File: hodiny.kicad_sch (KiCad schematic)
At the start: 58 parts, among them U1 DS1302+, U10 4511, U11 4511, U12 4511, U2 4511, U8 4511, U9 4511, Y1 32.768kHz

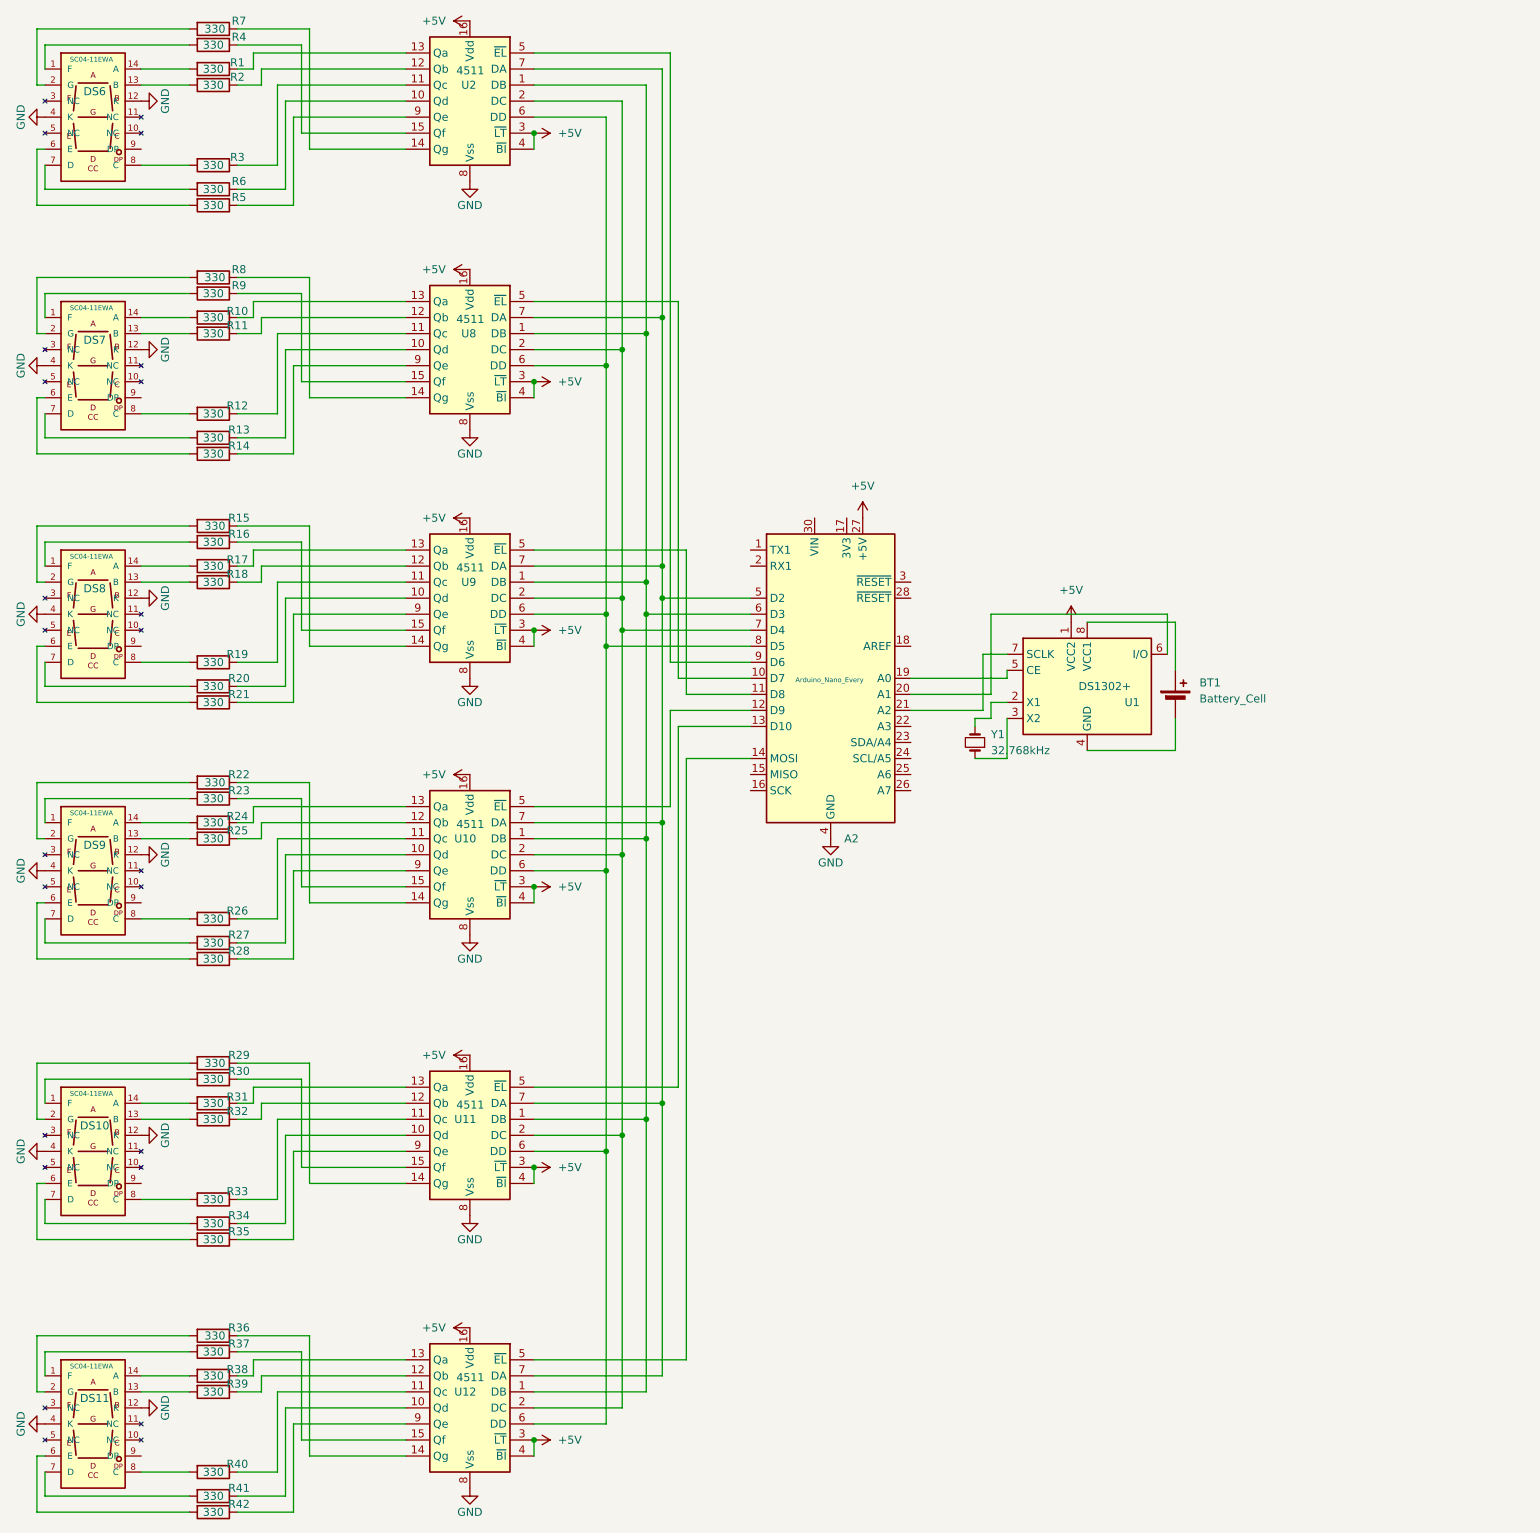
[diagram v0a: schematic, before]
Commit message: Add files via upload
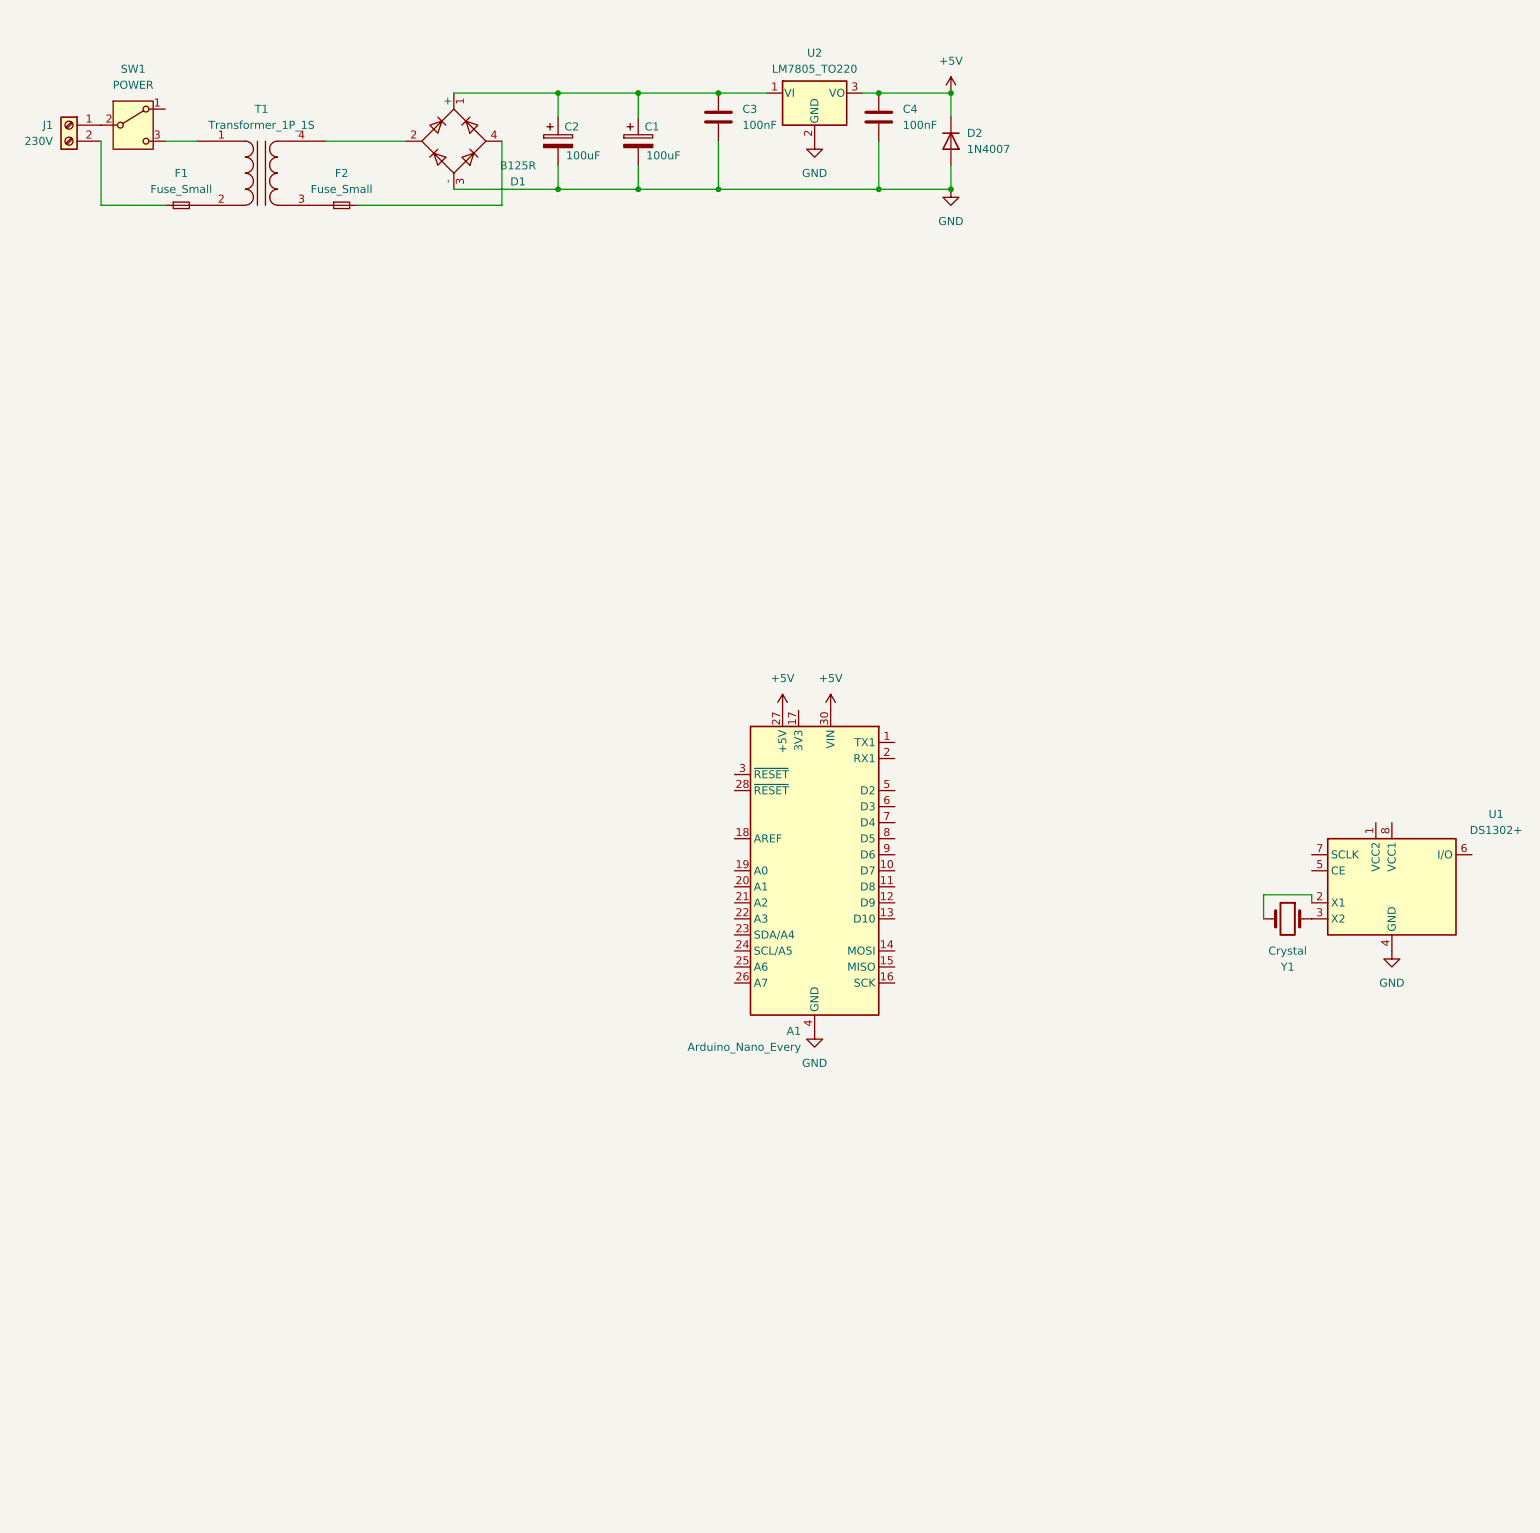
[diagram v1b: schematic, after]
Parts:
- removed A2: Arduino_Nano_Every, Module:Arduino_Nano, symbol MCU_Module:Arduino_Nano_Every
- removed BT1: Battery_Cell, Battery:BatteryHolder_ComfortableElectronic_CH273-2450_1x2450, symbol Device:Battery_Cell
- removed DS10, DS11, DS6, DS7, DS8, DS9: SC04-11EWA, SC04-11EWA:SC04-11EWA_THT, symbol SC04-11EWA:SC04-11EWA
- removed R1, R10, R11, R12, R13, R14, R15, R16, R17, R18, R19, R2, R20, R21, R22, R23, R24, R25, R26, R27, R28, R29, R3, R30, R31, R32, R33, R34, R35, R36, R37, R38, R39, R4, R40, R41, R42, R5, R6, R7, R8, R9: 330, Resistor_THT:R_Axial_DIN0411_L9.9mm_D3.6mm_P15.24mm_Horizontal, symbol Device:R
- removed U10, U11, U12, U2, U8, U9: 4511, Package_DIP:DIP-16_W7.62mm_Socket_LongPads, symbol 4xxx_IEEE:4511
- removed Y1: 32.768kHz, Crystal:Crystal_C26-LF_D2.1mm_L6.5mm_Horizontal, symbol PCM_SparkFun-Clock:Crystal_32.768kHz_3.2x1.5mm
- added A1: Arduino_Nano_Every, Module:Arduino_Nano, symbol MCU_Module:Arduino_Nano_Every
- added C1, C2: 100uF, Package_DFN_QFN:WDFN-10-1EP_3x3mm_P0.5mm_EP1.8x2.5mm, symbol Device:C_Polarized
- added C3, C4: 100nF, Diode_THT:Diode_Bridge_Round_D9.0mm, symbol Device:C
- added D1: B125R, Diode_THT:Diode_Bridge_Round_D9.0mm, symbol Diode_Bridge:B125R
- added D2: 1N4007, Diode_THT:D_DO-41_SOD81_P12.70mm_Horizontal, symbol Diode:1N4007
- added F1, F2: Fuse_Small, Package_QFP:LQFP-100_14x14mm_P0.5mm, symbol Device:Fuse_Small
- added J1: 230V, Package_DFN_QFN:QFN-20-1EP_5x5mm_P0.65mm_EP3.35x3.35mm, symbol Connector:Screw_Terminal_01x02
- added SW1: POWER, Button_Switch_THT:SW_NKK_GW12LJP, symbol Switch:SW_SPDT
- added T1: Transformer_1P_1S, symbol Device:Transformer_1P_1S
- added U2: LM7805_TO220, Package_TO_SOT_THT:TO-220-3_Vertical, symbol Regulator_Linear:LM7805_TO220
- added Y1: Crystal, Crystal:Crystal_AT310_D3.0mm_L10.0mm_Vertical, symbol Device:Crystal
- U1: footprint Package_DIP:DIP-8_W7.62mm_Socket_LongPads -> Package_DIP:DIP-8_W7.62mm_LongPads
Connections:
- net +5V: now also A1.27 (+5V), A1.30 (VIN), C4.1, D2.1 (K), U2.3 (VO); no longer U1.1 (VCC2)
- net GND: now also U1.4 (GND), A1.29 (GND), A1.4 (GND), C1.2, C2.2, C3.2, C4.2, D1.3 (-), D2.2 (A), U2.2 (GND)
- net at U1.2 (X1): now also Y1.2
- net at U1.3 (X2): now also Y1.1
- new net: C1.1, C2.1, C3.1, D1.1 (+), U2.1 (VI)
- new net: F1.1, J1.2 (Pin_2)
- new net: F1.2, T1.2 (AB)
- new net: J1.1 (Pin_1), SW1.2 (B)
- new net: SW1.3 (C), T1.1 (AA)
- new net: F2.1, T1.3 (SA)
- new net: D1.4, F2.2
- new net: D1.2, T1.4 (SB)

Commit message: Add files via upload
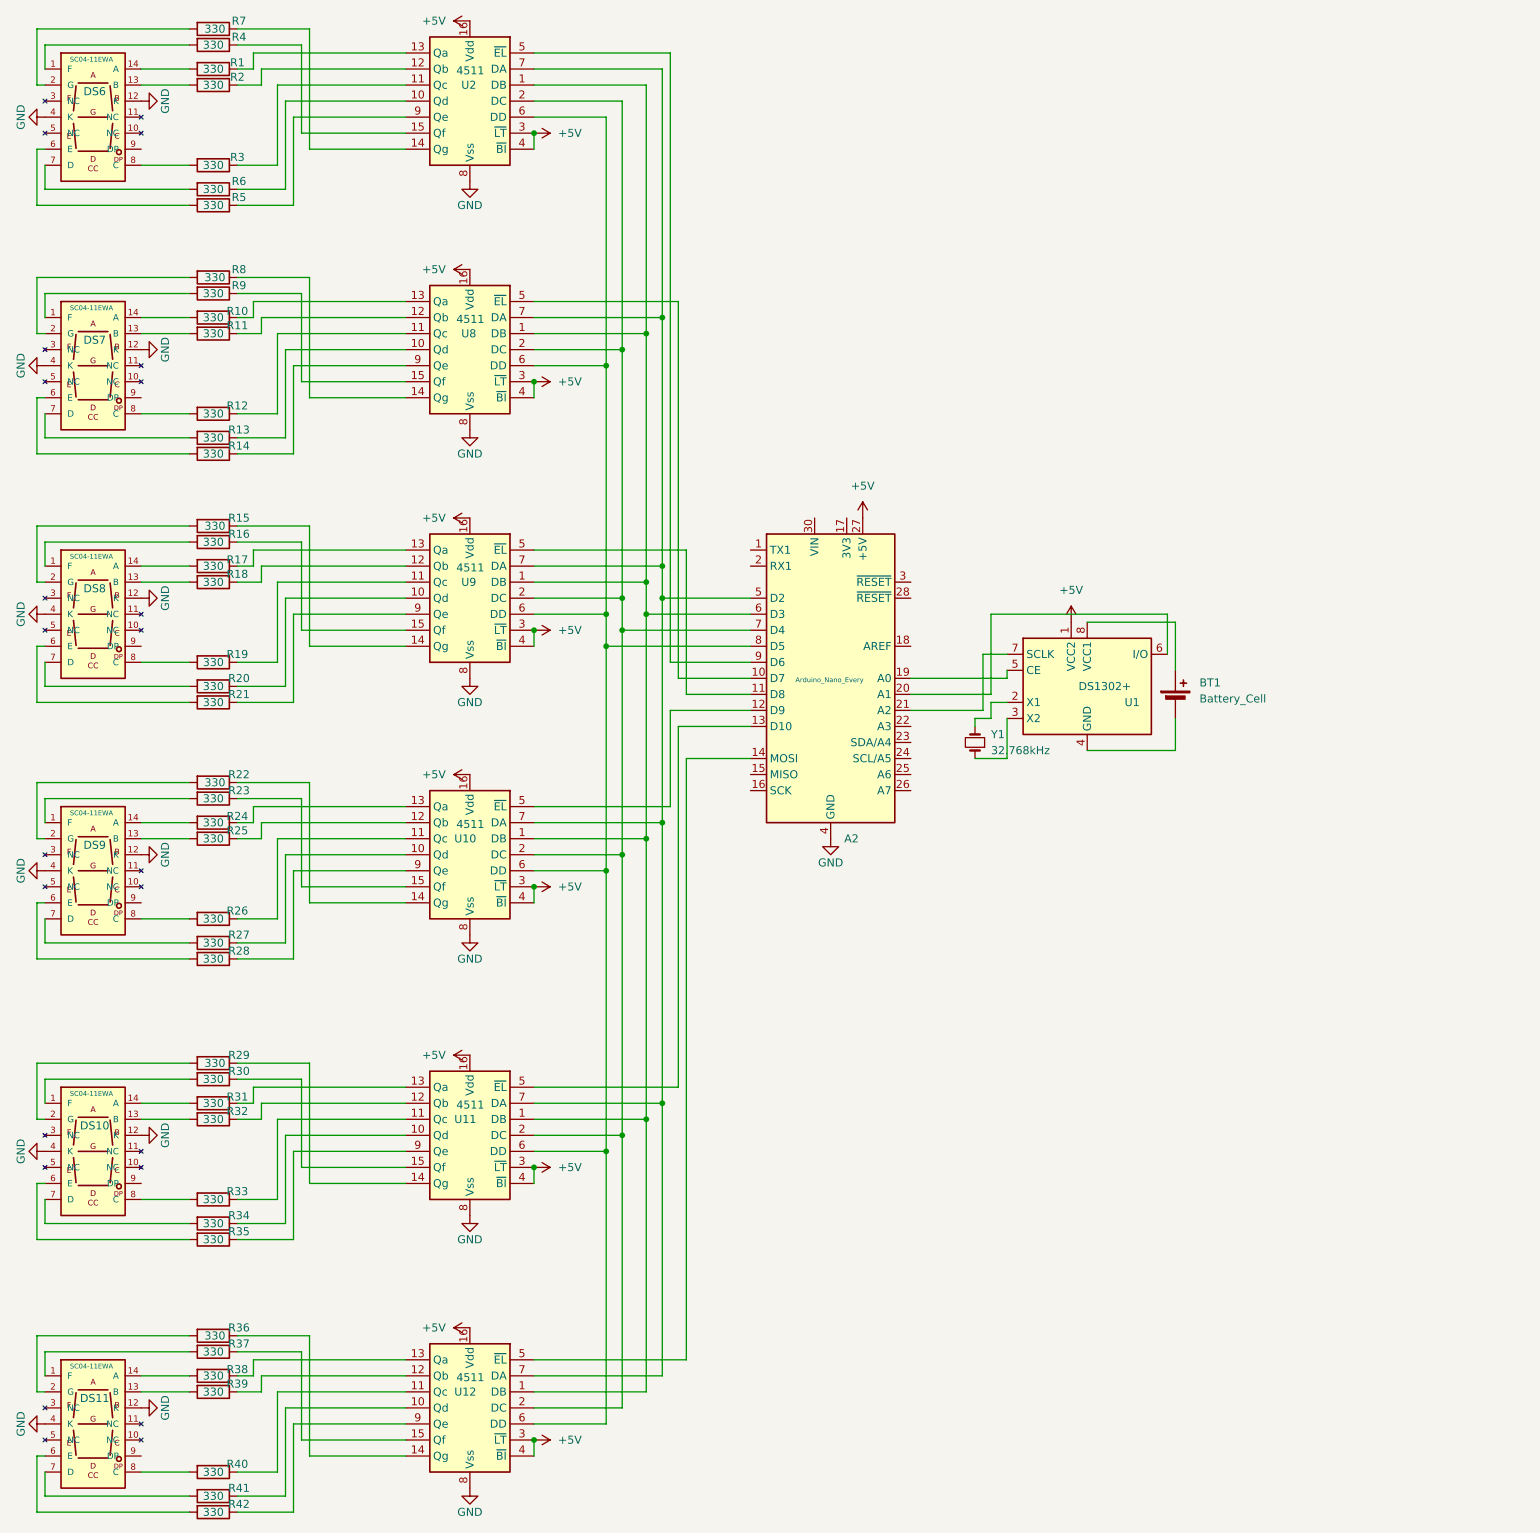
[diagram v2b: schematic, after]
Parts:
- removed A1: Arduino_Nano_Every, Module:Arduino_Nano, symbol MCU_Module:Arduino_Nano_Every
- removed C1, C2: 100uF, Package_DFN_QFN:WDFN-10-1EP_3x3mm_P0.5mm_EP1.8x2.5mm, symbol Device:C_Polarized
- removed C3, C4: 100nF, Diode_THT:Diode_Bridge_Round_D9.0mm, symbol Device:C
- removed D1: B125R, Diode_THT:Diode_Bridge_Round_D9.0mm, symbol Diode_Bridge:B125R
- removed D2: 1N4007, Diode_THT:D_DO-41_SOD81_P12.70mm_Horizontal, symbol Diode:1N4007
- removed F1, F2: Fuse_Small, Package_QFP:LQFP-100_14x14mm_P0.5mm, symbol Device:Fuse_Small
- removed J1: 230V, Package_DFN_QFN:QFN-20-1EP_5x5mm_P0.65mm_EP3.35x3.35mm, symbol Connector:Screw_Terminal_01x02
- removed SW1: POWER, Button_Switch_THT:SW_NKK_GW12LJP, symbol Switch:SW_SPDT
- removed T1: Transformer_1P_1S, symbol Device:Transformer_1P_1S
- removed U2: LM7805_TO220, Package_TO_SOT_THT:TO-220-3_Vertical, symbol Regulator_Linear:LM7805_TO220
- removed Y1: Crystal, Crystal:Crystal_AT310_D3.0mm_L10.0mm_Vertical, symbol Device:Crystal
- added A2: Arduino_Nano_Every, Module:Arduino_Nano, symbol MCU_Module:Arduino_Nano_Every
- added BT1: Battery_Cell, Battery:BatteryHolder_ComfortableElectronic_CH273-2450_1x2450, symbol Device:Battery_Cell
- added DS10, DS11, DS6, DS7, DS8, DS9: SC04-11EWA, SC04-11EWA:SC04-11EWA_THT, symbol SC04-11EWA:SC04-11EWA
- added R1, R10, R11, R12, R13, R14, R15, R16, R17, R18, R19, R2, R20, R21, R22, R23, R24, R25, R26, R27, R28, R29, R3, R30, R31, R32, R33, R34, R35, R36, R37, R38, R39, R4, R40, R41, R42, R5, R6, R7, R8, R9: 330, Resistor_THT:R_Axial_DIN0411_L9.9mm_D3.6mm_P15.24mm_Horizontal, symbol Device:R
- added U10, U11, U12, U2, U8, U9: 4511, Package_DIP:DIP-16_W7.62mm_Socket_LongPads, symbol 4xxx_IEEE:4511
- added Y1: 32.768kHz, Crystal:Crystal_C26-LF_D2.1mm_L6.5mm_Horizontal, symbol PCM_SparkFun-Clock:Crystal_32.768kHz_3.2x1.5mm
- U1: footprint Package_DIP:DIP-8_W7.62mm_LongPads -> Package_DIP:DIP-8_W7.62mm_Socket_LongPads
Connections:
- net +5V: now also U1.1 (VCC2), A2.27 (+5V), U10.16 (Vdd), U10.3 (~{LT}), U10.4 (~{BI}), U11.16 (Vdd), U11.3 (~{LT}), U11.4 (~{BI}), U12.16 (Vdd), U12.3 (~{LT}), U12.4 (~{BI}), U2.16 (Vdd), U2.3 (~{LT}), U2.4 (~{BI}), U8.16 (Vdd), U8.3 (~{LT}), U8.4 (~{BI}), U9.16 (Vdd), U9.3 (~{LT}), U9.4 (~{BI})
- net GND: now also A2.29 (GND), A2.4 (GND), DS10.12 (K), DS10.4 (K), DS11.12 (K), DS11.4 (K), DS6.12 (K), DS6.4 (K), DS7.12 (K), DS7.4 (K), DS8.12 (K), DS8.4 (K), DS9.12 (K), DS9.4 (K), U10.8 (Vss), U11.8 (Vss), U12.8 (Vss), U2.8 (Vss), U8.8 (Vss), U9.8 (Vss); no longer U1.4 (GND)
- net at U1.2 (X1): now also Y1.2
- net at U1.3 (X2): now also Y1.1
- net at U1.5 (CE): now also A2.19 (A0)
- net at U1.6 (I/O): now also A2.20 (A1)
- net at U1.7 (SCLK): now also A2.21 (A2)
- net at U1.8 (VCC1): now also BT1.1 (+)
- new net: DS7.1 (F), R9.2
- new net: DS7.13 (B), R11.2
- new net: DS7.14 (A), R10.2
- new net: DS7.2 (G), R8.2
- new net: DS7.6 (E), R14.2
- new net: DS7.7 (D), R13.2
- new net: DS7.8 (C), R12.2
- new net: R35.1, U11.9 (Qe)
- new net: DS10.6 (E), R35.2
- new net: R21.1, U9.9 (Qe)
- new net: DS8.6 (E), R21.2
- new net: R29.1, U11.14 (Qg)
- new net: DS10.2 (G), R29.2
- new net: R36.1, U12.14 (Qg)
- new net: DS11.2 (G), R36.2
- new net: R33.1, U11.11 (Qc)
- new net: DS10.8 (C), R33.2
- new net: R12.1, U8.11 (Qc)
- new net: DS6.1 (F), R4.2
- new net: DS6.13 (B), R2.2
- new net: DS6.14 (A), R1.2
- new net: DS6.2 (G), R7.2
- new net: DS6.6 (E), R5.2
- new net: DS6.7 (D), R6.2
- new net: DS6.8 (C), R3.2
- new net: R42.1, U12.9 (Qe)
- new net: DS11.6 (E), R42.2
- new net: R25.1, U10.12 (Qb)
- new net: DS9.13 (B), R25.2
- new net: R1.1, U2.13 (Qa)
- new net: R15.1, U9.14 (Qg)
- new net: DS8.2 (G), R15.2
- new net: R14.1, U8.9 (Qe)
- new net: DS9.1 (F), R23.2
- new net: DS9.14 (A), R24.2
- new net: DS9.2 (G), R22.2
- new net: DS9.6 (E), R28.2
- new net: DS9.7 (D), R27.2
- new net: DS9.8 (C), R26.2
- new net: R22.1, U10.14 (Qg)
- new net: R11.1, U8.12 (Qb)
- new net: A2.6 (D3), U10.1 (DB), U11.1 (DB), U12.1 (DB), U2.1 (DB), U8.1 (DB), U9.1 (DB)
- new net: R34.1, U11.10 (Qd)
- new net: R32.1, U11.12 (Qb)
- new net: R31.1, U11.13 (Qa)
- new net: R30.1, U11.15 (Qf)
- new net: A2.7 (D4), U10.2 (DC), U11.2 (DC), U12.2 (DC), U2.2 (DC), U8.2 (DC), U9.2 (DC)
- new net: A2.13 (D10), U11.5 (~{EL})
- new net: A2.8 (D5), U10.6 (DD), U11.6 (DD), U12.6 (DD), U2.6 (DD), U8.6 (DD), U9.6 (DD)
- new net: A2.5 (D2), U10.7 (DA), U11.7 (DA), U12.7 (DA), U2.7 (DA), U8.7 (DA), U9.7 (DA)
- new net: R16.1, U9.15 (Qf)
- new net: DS8.1 (F), R16.2
- new net: R19.1, U9.11 (Qc)
- new net: DS8.8 (C), R19.2
- new net: R38.1, U12.13 (Qa)
- new net: DS11.14 (A), R38.2
- new net: A2.10 (D7), U8.5 (~{EL})
- new net: A2.11 (D8), U9.5 (~{EL})
- new net: A2.12 (D9), U10.5 (~{EL})
- new net: A2.14 (MOSI), U12.5 (~{EL})
- new net: A2.9 (D6), U2.5 (~{EL})
- new net: R41.1, U12.10 (Qd)
- new net: DS11.7 (D), R41.2
- new net: R20.1, U9.10 (Qd)
- new net: DS8.7 (D), R20.2
- new net: R27.1, U10.10 (Qd)
- new net: R26.1, U10.11 (Qc)
- new net: R24.1, U10.13 (Qa)
- new net: R23.1, U10.15 (Qf)
- new net: R28.1, U10.9 (Qe)
- new net: R10.1, U8.13 (Qa)
- new net: R2.1, U2.12 (Qb)
- new net: DS11.1 (F), R37.2
- new net: DS11.13 (B), R39.2
- new net: DS11.8 (C), R40.2
- new net: R3.1, U2.11 (Qc)
- new net: R39.1, U12.12 (Qb)
- new net: R7.1, U2.14 (Qg)
- new net: BT1.2 (-), U1.4 (GND)
- new net: DS10.7 (D), R34.2
- new net: R13.1, U8.10 (Qd)
- new net: R8.1, U8.14 (Qg)
- new net: R9.1, U8.15 (Qf)
- new net: DS10.1 (F), R30.2
- new net: DS10.13 (B), R32.2
- new net: DS10.14 (A), R31.2
- new net: R18.1, U9.12 (Qb)
- new net: DS8.13 (B), R18.2
- new net: R6.1, U2.10 (Qd)
- new net: R4.1, U2.15 (Qf)
- new net: R5.1, U2.9 (Qe)
- new net: R37.1, U12.15 (Qf)
- new net: DS8.14 (A), R17.2
- new net: R17.1, U9.13 (Qa)
- new net: R40.1, U12.11 (Qc)
